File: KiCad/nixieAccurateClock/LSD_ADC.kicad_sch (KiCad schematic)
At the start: 13 parts, among them U11 TXB0108PWR, U12 TXB0108PWR

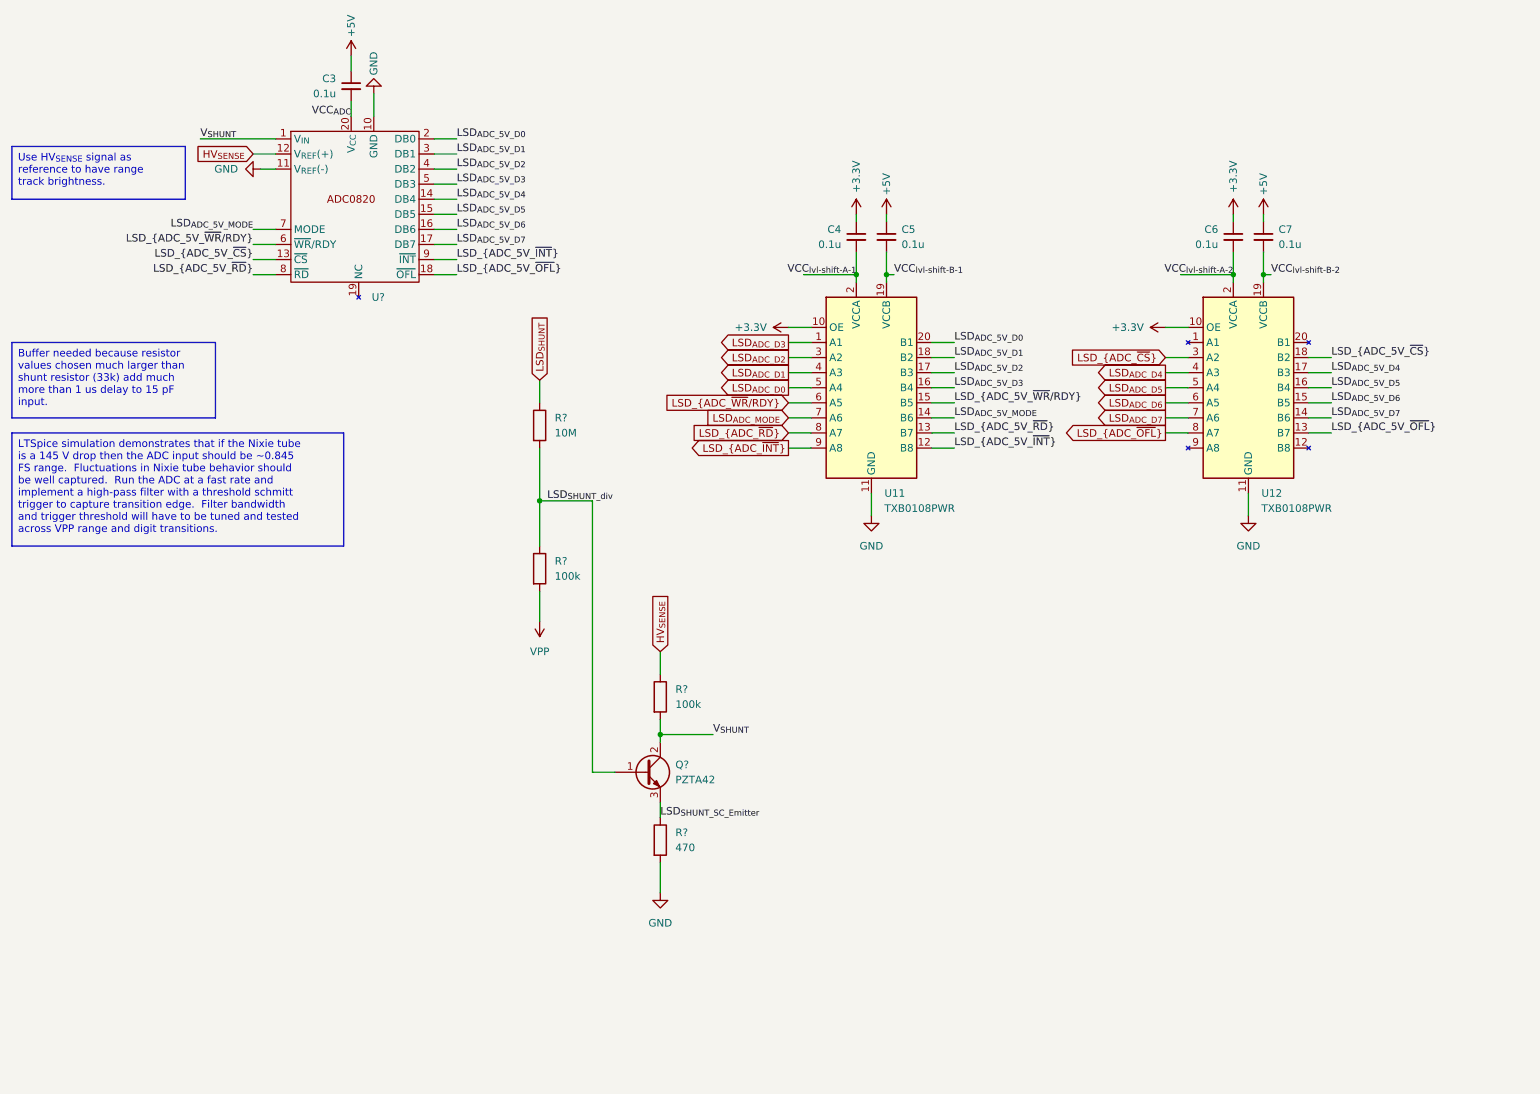
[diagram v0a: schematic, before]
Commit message: add delay resistor to level shifter OE
Resistor is shown on TX0108 data sheet.
Likely helps slow OE with capacitive input to help with power-on sequencing.
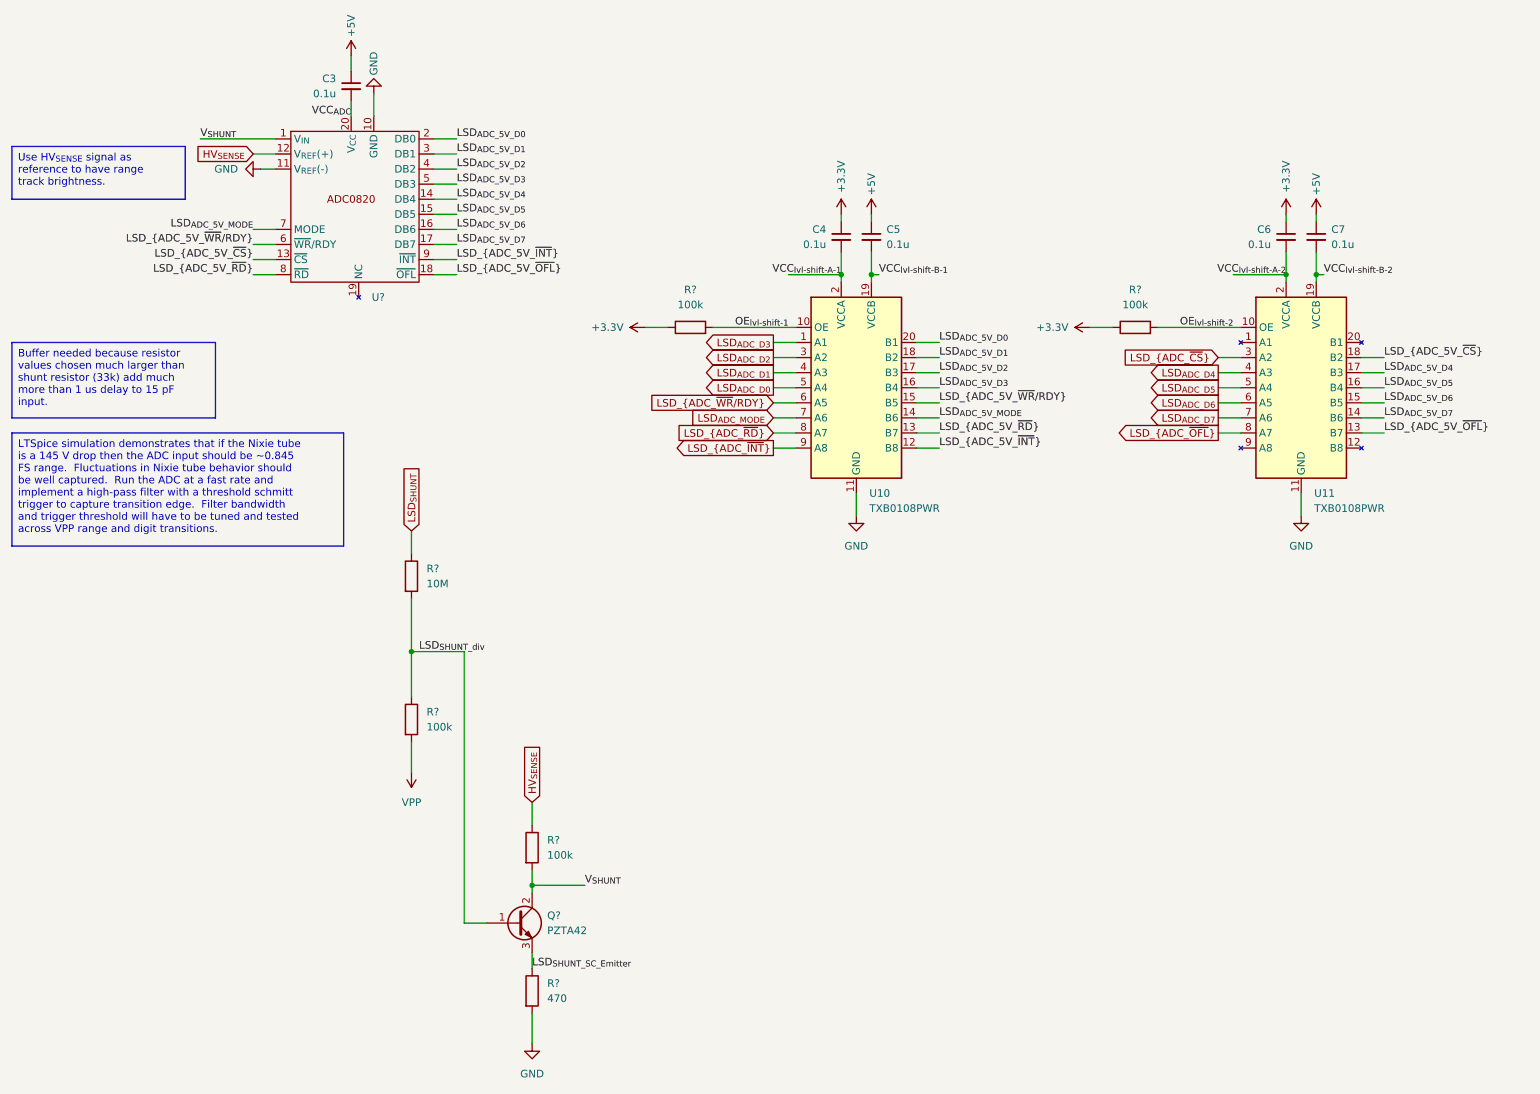
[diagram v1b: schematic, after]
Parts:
- added R? (x2): 100k, Resistor_SMD:R_0603_1608Metric, symbol Device:R
- renumbered U11 to U10, U12 to U11
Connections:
- net +3.3V: now also R?.1, R?.1; no longer U10.10 (OE), U11.10 (OE)
- new net OE_{lvl-shift-1}: R?.2, U10.10 (OE)
- new net OE_{lvl-shift-2}: R?.2, U11.10 (OE)
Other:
- moved on the sheet: C4, C5, C6, C7, Q?, R?, U10, U11
